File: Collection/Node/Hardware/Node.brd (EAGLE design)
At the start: 41.9 x 68.6 mm, 20 parts, among them IC1 4050D, IC2 LP298XS, IC3 DS3231/SO, M2 WIRELESS-NRF24L01-PA-EXT, Q1 16MHz, SW2 FSMSM, U2 ATMEGA328P-PU, X1 MICROSD

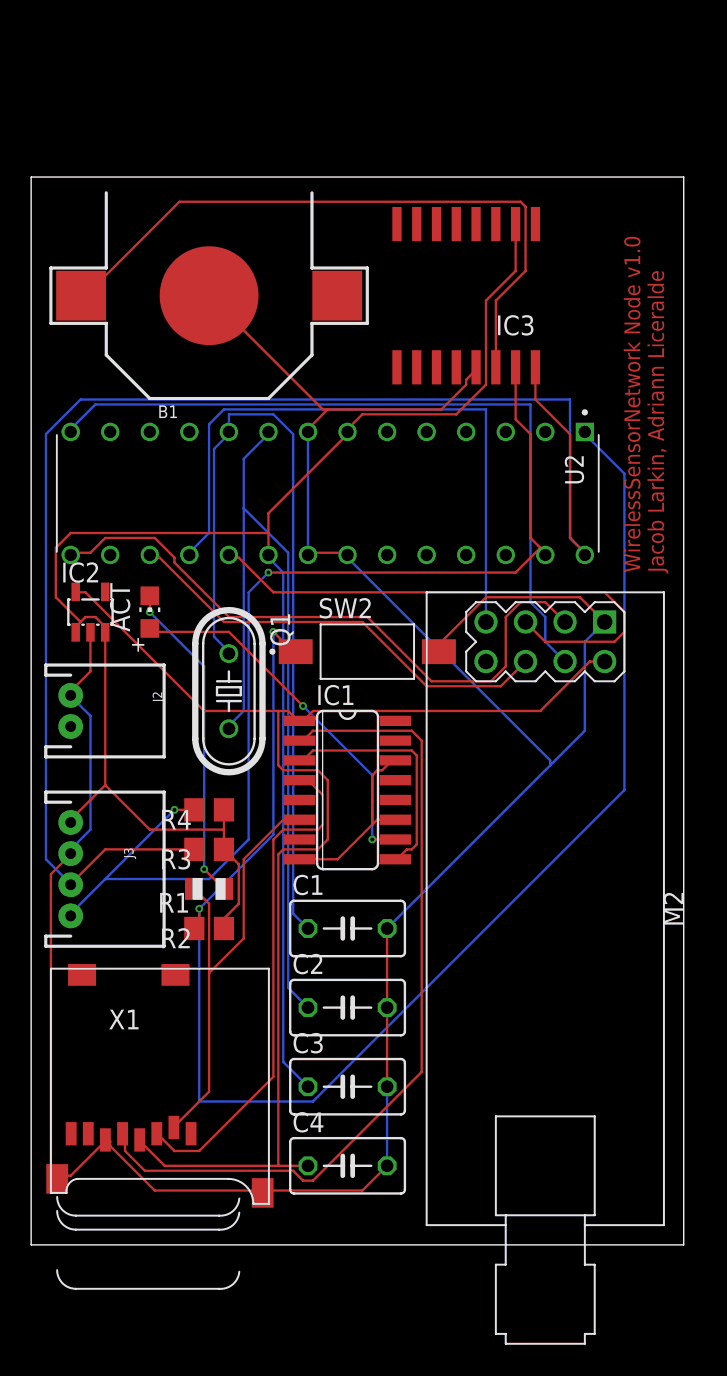
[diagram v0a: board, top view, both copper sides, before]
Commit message: updated schematic
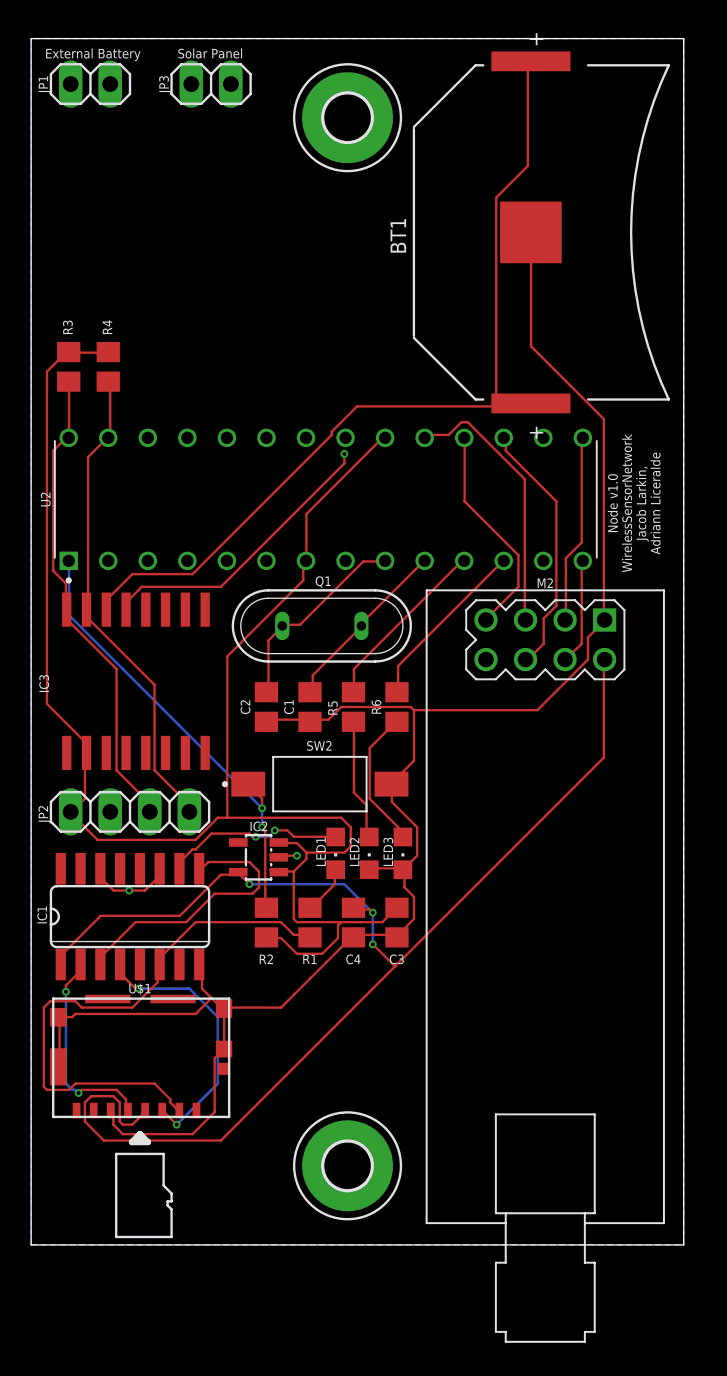
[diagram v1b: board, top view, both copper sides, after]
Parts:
- removed ACT: RED, adafruit:CHIP-LED0805
- removed B1: CR1220, microbuilder:CR1220
- removed J2: (no value), SparkFun-Connectors:JST-2-PTH
- removed J3: (no value), SparkFun-Connectors:JST-4-PTH
- removed X1: MICROSD, adafruit:MICROSD
- added BT1: KEYSTONE_ELECTRONICS_3034KEYSTONE_ELECTRONICS_3034_0_0, Keystone Electronics - 3034:KEYSTONE_ELECTRONICS_3034_0
- added H1, H2: MOUNT-PAD-ROUND3.0, holes:3,0-PAD
- added JP1, JP3: (no value), pinhead:1X02
- added JP2: (no value), pinhead:1X04
- added LED1: RED, led:CHIPLED_0805
- added LED2: GREEN, led:CHIPLED_0805
- added LED3: Yellow, led:CHIPLED_0805
- added R5, R6: 1K, rcl:R0805
- added U$1: 1051620001A, Molex_micro_SD:1051620001_SMT
- C1, C2, C3, C4: device rcl:C050-035X075 -> rcl:C0805
- Q1: device crystal:HC49/S -> special:QS
- R1: device adafruit:R0805 -> rcl:R0805
- moved IC3 32.6 mm to (6.73, 36.2), turned to 0 degrees
- moved R3 32.3 mm to (2.41, 56.4), turned to 90 degrees
- moved R4 29.2 mm to (4.95, 56.4), turned to 90 degrees
- moved C2 20.0 mm to (15.1, 34.5), turned to 270 degrees
- moved IC2 19.1 mm to (14.6, 24.9), turned to 90 degrees
- moved IC1 16.2 mm to (6.35, 21.1), turned to 0 degrees
- moved C4 15.6 mm to (20.7, 20.7), turned to 270 degrees
- moved C1 14.4 mm to (17.9, 34.5), turned to 270 degrees
- moved C3 11.0 mm to (23.5, 20.7), turned to 270 degrees
- moved SW2 9.04 mm to (18.5, 29.6)
- moved Q1 7.29 mm to (18.7, 39.8), turned to 180 degrees
- moved R1 6.83 mm to (17.9, 20.7), turned to 90 degrees
- moved R2 3.70 mm to (15.1, 20.7), turned to 270 degrees
- moved U2 0.40 mm to (18.9, 47.9), turned to 90 degrees
- moved M2 0.13 mm to (33.0, 21.7)
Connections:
- removed net CD: X1.CD1
- removed net GND_SD: IC1.11, IC1.14, IC1.8
- removed net V_EXTERNAL_BATTERY: J2.2
- new net N$10: LED2.A, R5.1
- new net N$11: LED3.A, R6.1
- new net N$12: R6.2, U2.12
- new net N$9: R5.2, U2.11
- new net V_PACK: JP1.1
- net +3V3: now also U$1.4; no longer X1.4
- net +5V: now also JP2.4; no longer J3.1
- net DO: now also U$1.7; no longer X1.7
- net GND: now also BT1.1, IC1.11, IC1.14, IC1.8, JP1.2, JP2.3, JP3.2, LED2.C, LED3.C, U$1.6, U$1.G1, U$1.G2, U$1.G3, U$1.G4; no longer B1.-, J2.1, J3.2, X1.6, X1.MT1, X1.MT2
- net N$1: now also LED1.A; no longer ACT.A
- net N$2: now also U$1.5; no longer X1.5
- net N$3: now also U$1.2; no longer X1.2
- net N$4: now also LED1.C; no longer ACT.C
- net N$5: now also U$1.3; no longer X1.3
- net SCL: now also JP2.2; no longer J3.3
- net SDA: now also JP2.1; no longer J3.4
- net VBAT: now also BT1.2, BT1.2-2; no longer B1.+$1
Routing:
- net SCL: track 96.8 -> 30.7 mm
- net N$6: track 95.3 -> 29.4 mm
- net N$7: track 53.0 -> 11.6 mm
- net CSN: track 47.8 -> 6.86 mm
- net N$8: track 53.9 -> 13.0 mm
- net N$2: track 53.5 -> 13.3 mm, vias 0 -> 2
- net SDA: track 70.3 -> 31.1 mm, vias 2 -> 0
- net CE: track 40.8 -> 12.2 mm
- net MISO: track 40.7 -> 14.0 mm
- net GND: track 168.9 -> 142.8 mm, vias 0 -> 3
- net SCK: track 35.4 -> 17.4 mm
- net N$4: track 20.9 -> 3.15 mm, vias 2 -> 0
- net VBAT: track 42.3 -> 58.6 mm
- net N$5: track 32.5 -> 17.3 mm, vias 0 -> 2
- net N$1: track 23.9 -> 11.6 mm
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- added copper zone on layer 16, net GND
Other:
- board size 41.9 x 68.6 mm -> 41.9 x 77.5 mm
- board text added: "External Battery"
- board text added: "Node v1.0 WirelessSensorNetwork Jacob Larkin, Adriann Liceralde"
- board text added: "Solar Panel"
- board text removed: "WirelessSensorNetwork Node v1.0 Jacob Larkin, Adriann Liceralde"
